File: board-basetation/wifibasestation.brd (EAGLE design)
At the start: 50 x 22 mm, 33 parts, among them IC1 1117EMP, IC2 HTU21D, J1 SWD_SHROUD_SMD, X1 ESP-03, X2 SMA-142-0711-821/826

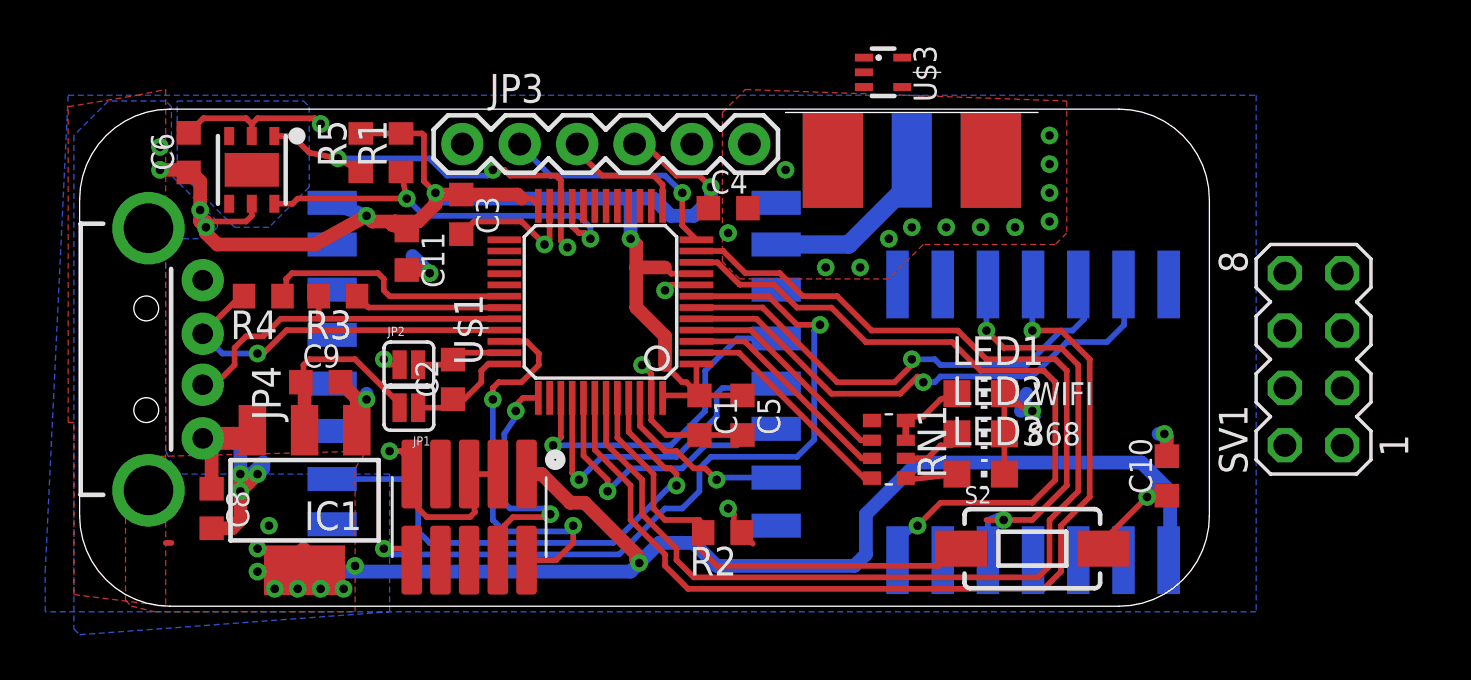
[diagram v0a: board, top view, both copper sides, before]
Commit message: something changed probably
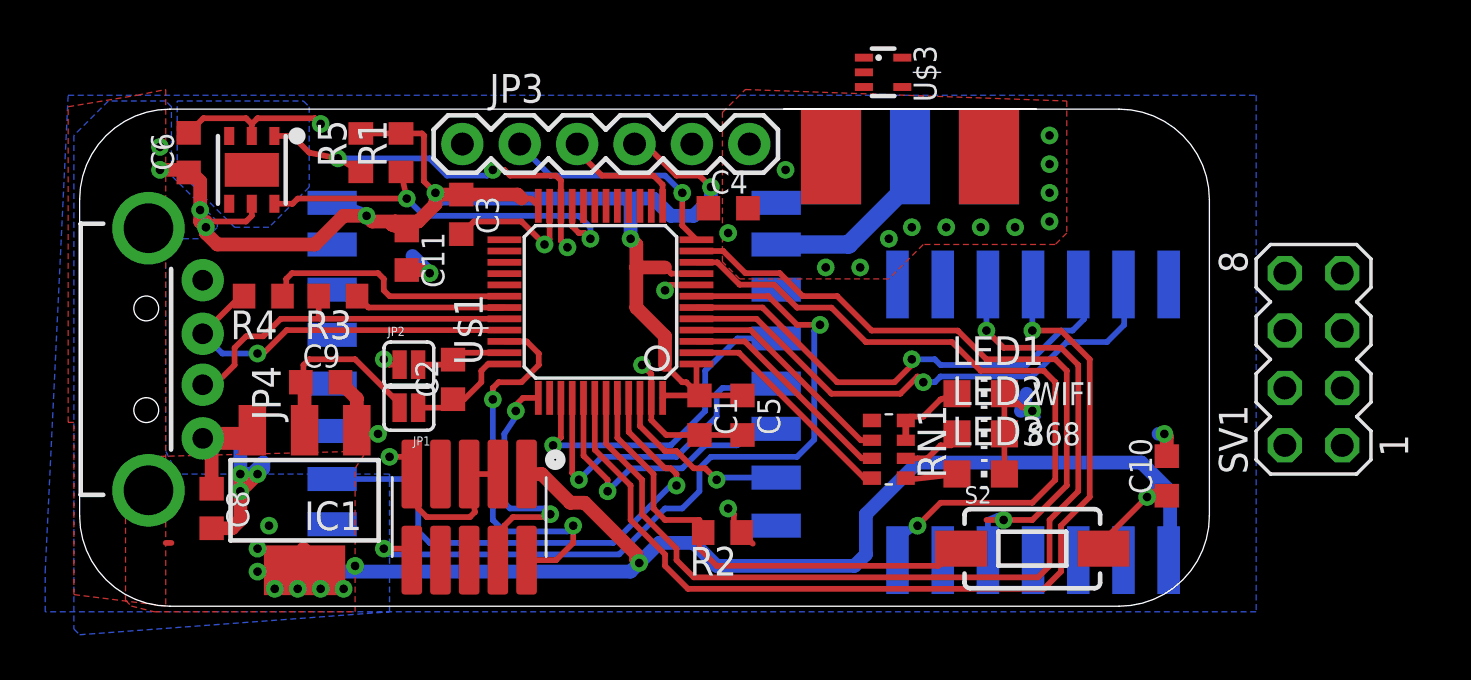
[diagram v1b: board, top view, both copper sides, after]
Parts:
- moved X2 0.17 mm to (36.8, 22.5)
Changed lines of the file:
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@@
 <element name="C6" library="rcl" package="C0603K" value="" x="4.826" y="20.574" rot="R90"/>
 <element name="X1" library="Mine" package="ESP-03" value="ESP-03" x="34.798" y="2.54" rot="MR0"/>
-<element name="X2" library="con-coax" package="J502-ND-142-0711-821/826" value="SMA-142-0711-821/826" x="36.83" y="22.352" rot="MR270">
-<attribute name="OC_NEWARK" value="16F3627" x="36.83" y="22.352" size="1.778" layer="28" rot="MR270" display="off"/>
-<attribute name="MPN" value="142-0711-821" x="36.83" y="22.352" size="1.778" layer="28" rot="MR270" display="off"/>
-<attribute name="MF" value="JOHNSON COMPONENTS" x="36.83" y="22.352" size="1.778" layer="28" rot="MR270" display="off"/>
-<attribute name="OC_FARNELL" value="1019328" x="36.83" y="22.352" size="1.778" layer="28" rot="MR270" display="off"/>
+<element name="X2" library="con-coax" package="J502-ND-142-0711-821/826" value="SMA-142-0711-821/826" x="36.75" y="22.5" rot="MR270">
+<attribute name="OC_NEWARK" value="16F3627" x="36.75" y="22.5" size="1.778" layer="28" rot="MR270" display="off"/>
+<attribute name="MPN" value="142-0711-821" x="36.75" y="22.5" size="1.778" layer="28" rot="MR270" display="off"/>
+<attribute name="MF" value="JOHNSON COMPONENTS" x="36.75" y="22.5" size="1.778" layer="28" rot="MR270" display="off"/>
+<attribute name="OC_FARNELL" value="1019328" x="36.75" y="22.5" size="1.778" layer="28" rot="MR270" display="off"/>
 </element>
 <element name="S2" library="SparkFun-Electromechanical" package="TACTILE-SWITCH-1101NE" value="SWITCH-MOMENTARY-2SMD-1101NE" x="42.164" y="3.048">
@@
 <via x="15.494" y="15.24" extent="1-16" drill="0.381" shape="octagon"/>
 <wire x1="15.494" y1="15.24" x2="14.732" y2="16.002" width="0.6096" layer="16"/>
-<wire x1="12.2674" y1="8.2888" x2="12.2674" y2="9.2194" width="0.6096" layer="1"/>
-<wire x1="12.2674" y1="9.2194" x2="12.7" y2="9.652" width="0.6096" layer="1"/>
-<via x="12.7" y="9.652" extent="1-16" drill="0.381" shape="octagon"/>
-<wire x1="12.7" y1="9.652" x2="12.7" y2="9.906" width="0.6096" layer="16"/>
-<wire x1="12.2674" y1="9.2194" x2="12.2674" y2="9.6896" width="0.6096" layer="1"/>
+<wire x1="12.2674" y1="8.2888" x2="12.2674" y2="9.6896" width="0.6096" layer="1"/>
+<via x="13.208" y="8.128" extent="1-16" drill="0.381" shape="octagon"/>
 <wire x1="12.2674" y1="9.6896" x2="11.543" y2="10.414" width="0.6096" layer="1"/>
 <wire x1="5.842" y1="3.951" x2="6.745" y2="3.951" width="0.6096" layer="1"/>
@@
 <wire x1="7.112" y1="6.35" x2="7.112" y2="7.874" width="0.6096" layer="16"/>
 <wire x1="7.112" y1="6.35" x2="7.112" y2="5.588" width="0.6096" layer="16"/>
-<via x="13.716" y="7.366" extent="1-16" drill="0.381" shape="octagon"/>
+<via x="13.716" y="7.112" extent="1-16" drill="0.381" shape="octagon"/>
 <via x="7.874" y="6.35" extent="1-16" drill="0.381" shape="octagon"/>
 <wire x1="7.112" y1="6.35" x2="7.62" y2="6.35" width="0.6096" layer="16"/>
@@
 <wire x1="8.128" y1="6.604" x2="7.874" y2="6.35" width="0.6096" layer="16"/>
 <wire x1="7.112" y1="5.588" x2="7.874" y2="6.35" width="0.6096" layer="1"/>
-<wire x1="13.716" y1="7.366" x2="14.224" y2="7.366" width="0.254" layer="1"/>
-<wire x1="14.224" y1="7.366" x2="14.478" y2="7.112" width="0.254" layer="1"/>
+<wire x1="13.716" y1="7.112" x2="14.478" y2="7.112" width="0.254" layer="1"/>
 <wire x1="14.478" y1="7.112" x2="14.478" y2="6.572" width="0.254" layer="1"/>
 <wire x1="14.478" y1="6.572" x2="14.7" y2="6.35" width="0.254" layer="1"/>
@@
 <vertex x="29.464" y="23.368"/>
 </polygon>
+<wire x1="13.208" y1="8.128" x2="12.4282" y2="8.128" width="0.254" layer="1"/>
+<wire x1="12.4282" y1="8.128" x2="12.2674" y2="8.2888" width="0.254" layer="1"/>
 <wire x1="48.006" y1="8.128" x2="55.88" y2="15.24" width="0" layer="19" extent="16-16"/>
 </signal>
@@
 <wire x1="5.588" y1="17.018" x2="6.096" y2="16.51" width="0.6096" layer="1"/>
 <wire x1="6.096" y1="16.51" x2="10.414" y2="16.51" width="0.6096" layer="1"/>
-<wire x1="10.414" y1="16.51" x2="12.7" y2="17.78" width="0.6096" layer="1"/>
 <via x="3.556" y="19.812" extent="1-16" drill="0.381" shape="octagon"/>
 <wire x1="3.556" y1="19.812" x2="4.826" y2="19.812" width="0.6096" layer="1"/>
@@
 <wire x1="25.908" y1="11.176" x2="26.67" y2="10.414" width="0.254" layer="1"/>
 <wire x1="48.26" y1="5.588" x2="53.34" y2="7.62" width="0" layer="19" extent="16-16"/>
+<wire x1="12.7" y1="17.78" x2="11.684" y2="17.78" width="0.6096" layer="1"/>
+<wire x1="11.684" y1="17.78" x2="10.414" y2="16.51" width="0.6096" layer="1"/>
 </signal>
 <signal name="N$15">
@@
 <wire x1="34.03625" y1="16.51025" x2="36.576" y2="19.05" width="0.8128" layer="16"/>
 <wire x1="36.576" y1="19.05" x2="36.576" y2="19.9826" width="0.8128" layer="16"/>
-<wire x1="36.576" y1="19.9826" x2="36.83" y2="20.2366" width="0.8128" layer="16"/>
+<wire x1="36.576" y1="19.9826" x2="36.75" y2="20.3846" width="0.8128" layer="16"/>
 </signal>
 <signal name="N$19">
